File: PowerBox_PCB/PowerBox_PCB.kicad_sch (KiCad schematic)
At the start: 3 parts

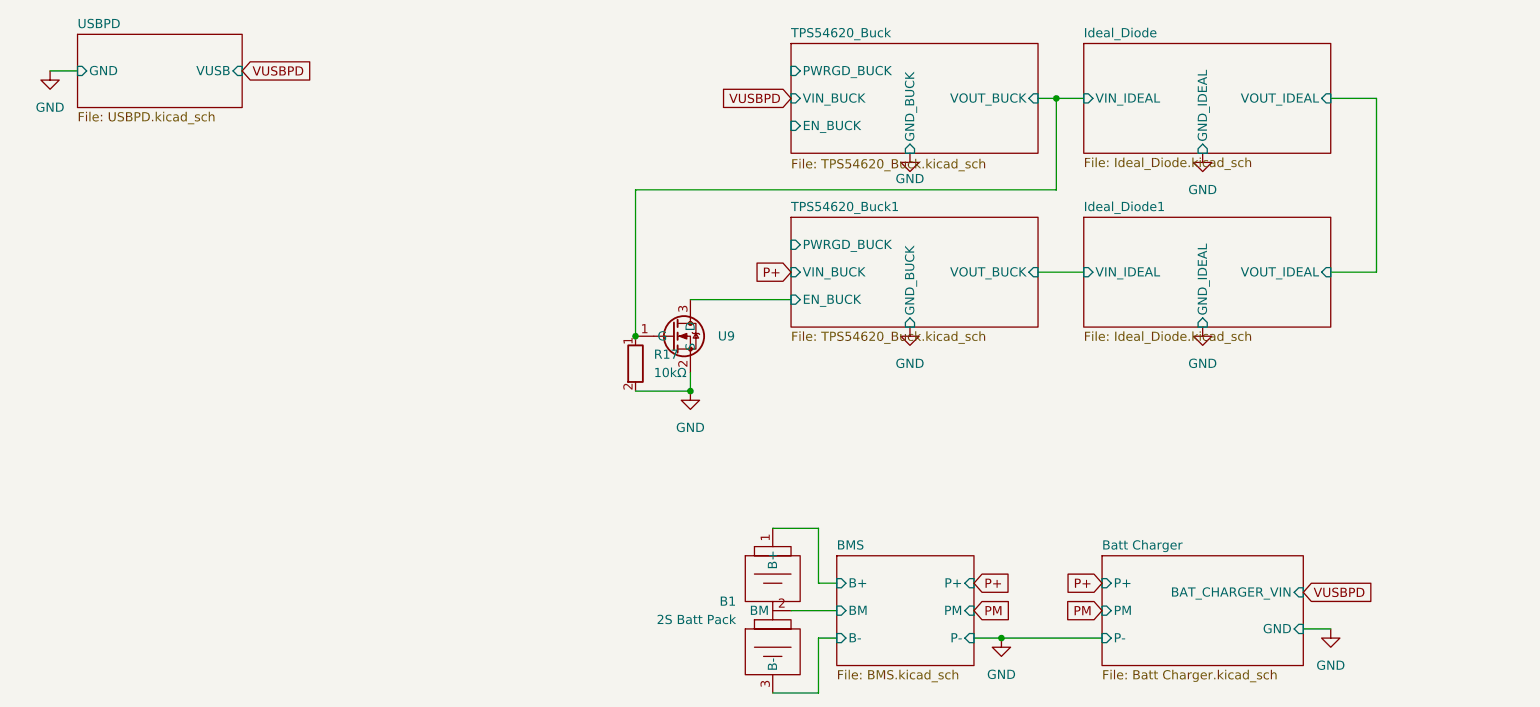
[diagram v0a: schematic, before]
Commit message: Finished
Basically done
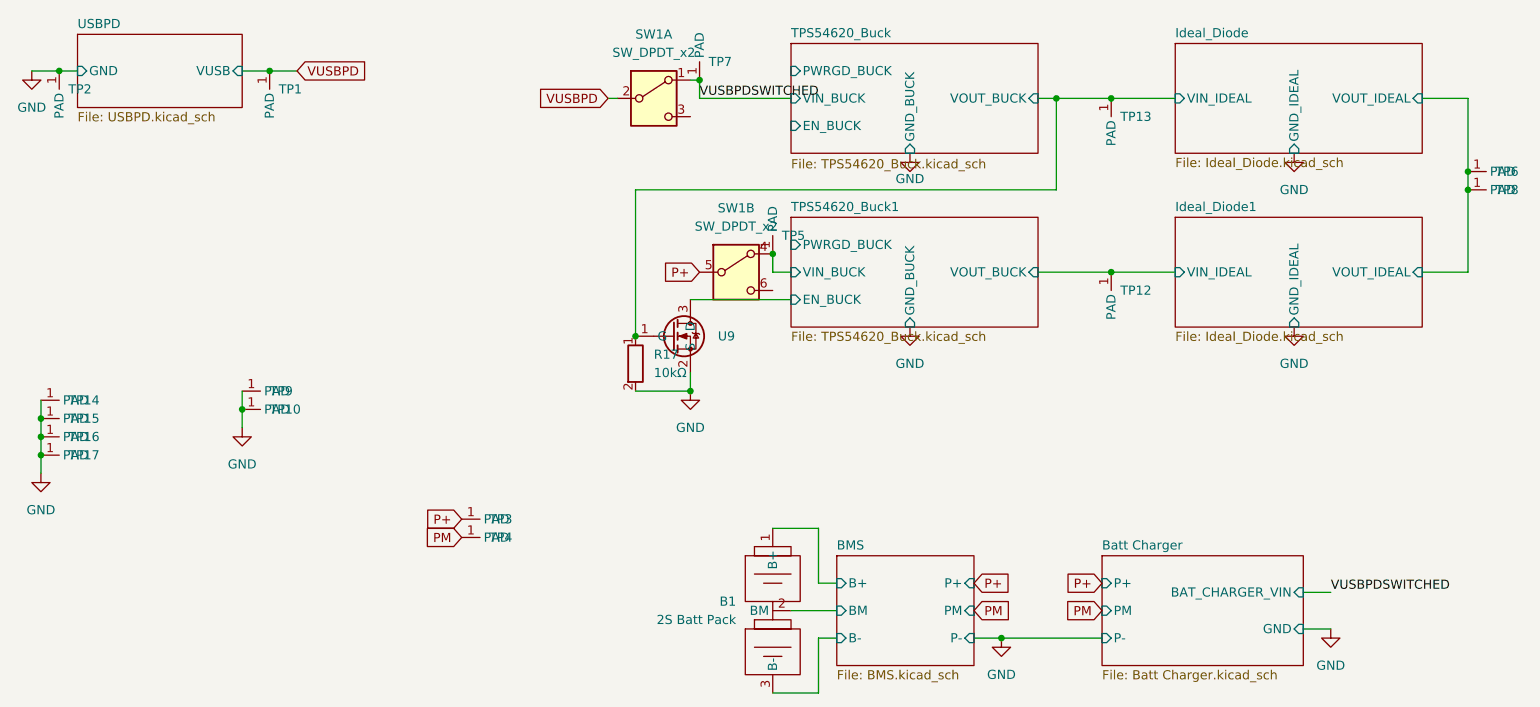
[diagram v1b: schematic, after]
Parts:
- added SW1: SW_DPDT_x2, Custom_Footprints:SwitchPads, symbol BMS:SW_DPDT_x2
- added TP1, TP10, TP12, TP13, TP2, TP3, TP4, TP5, TP6, TP7, TP8, TP9: (no value), Custom_Footprints:PAD-2x2, symbol Custom_Symbols:Pad-2x2
- added TP14, TP15, TP16, TP17: (no value), Custom_Footprints:M3-Pad, symbol Custom_Symbols:M3-PAD
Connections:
- net GND: now also TP10.1 (PAD), TP14.1 (PAD), TP15.1 (PAD), TP16.1 (PAD), TP17.1 (PAD), TP2.1 (PAD), TP9.1 (PAD)
- net Ideal_Diode/VIN_IDEAL: now also TP13.1 (PAD)
- net Ideal_Diode/VOUT_IDEAL: now also TP6.1 (PAD), TP8.1 (PAD)
- net Ideal_Diode1/VIN_IDEAL: now also TP12.1 (PAD)
- net P+: now also SW1.5 (B), TP3.1 (PAD)
- net PM: now also TP4.1 (PAD)
- net VUSBPD: now also SW1.2 (B), TP1.1 (PAD)
- new net TPS54620_Buck1/VIN_BUCK: SW1.4 (A), TP5.1 (PAD)
- new net VUSBPDSWITCHED: SW1.1 (A), TP7.1 (PAD)
